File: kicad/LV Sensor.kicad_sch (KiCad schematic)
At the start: 69 parts, among them IC1 MCP2517FDT-H_SL, IC2 L78L05ABUTR, IC3 TLV74133PDBVR, IC4 TLV74125PDBVR, J1 Screw_Terminal_01x02, J16 USB_B_Micro, J2 Screw_Terminal_01x02, J3 Screw_Terminal_01x02, J4 Screw_Terminal_01x02, J5 Screw_Terminal_01x02, J6 Screw_Terminal_01x02, SW1 SW_Push, U0 AP63205WU-7, U10 MCP3204-CI/P, U2 XMSM0C1104SPW20R, U3 FT231XS-R, U6 DSC1001DL5-020.0000T, U7 ADS114S06BIPBSR, U8 LM2662MX/NOPB, U9 ATA6561-GAQW-N

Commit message: dfggd
fd
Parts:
- removed J6: Screw_Terminal_01x02, TerminalBlock_MetzConnect:TerminalBlock_MetzConnect_Type059_RT06302HBWC_1x02_P3.50mm_Horizontal, symbol Connector:Screw_Terminal_01x02
- added J6: 43650-0415, ADC2_AND_4:43650-04YY_151617, symbol LV-Sensor-Lib:43650-0415
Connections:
- net +12V: now also J6.1
- net GND: now also J6.2
- net CAN_L: now reaches U9.6 (CANL)
- net CAN_L: now also J6.4
- net CAN_H: now reaches U9.7 (CANH)
- net CAN_H: now also J6.3

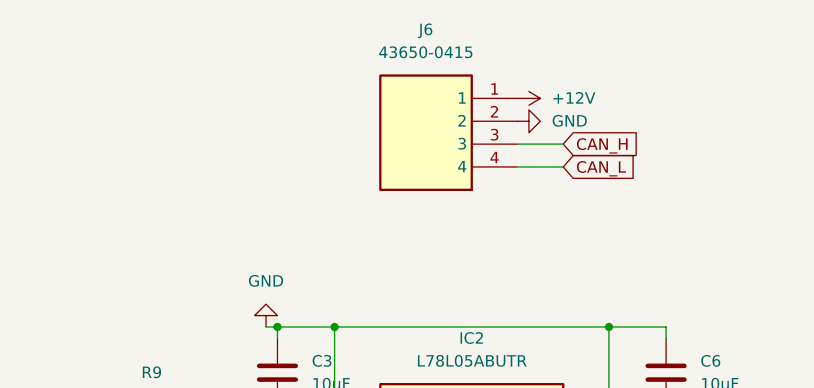
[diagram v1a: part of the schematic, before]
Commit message: fdg
dgf
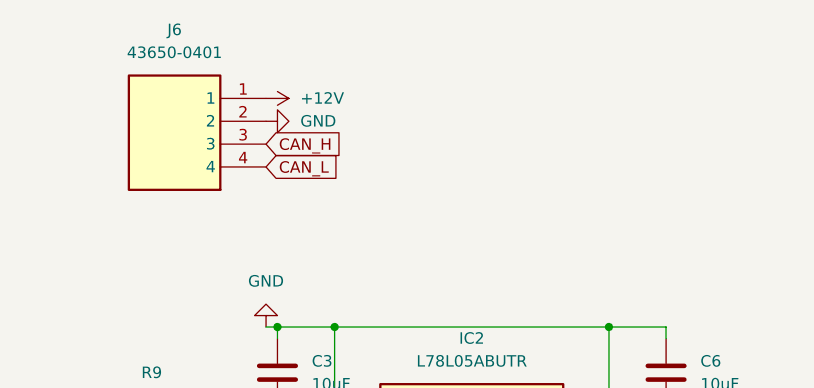
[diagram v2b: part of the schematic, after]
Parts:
- removed J6: 43650-0415, ADC2_AND_4:43650-04YY_151617, symbol LV-Sensor-Lib:43650-0415
- added J6: 43650-0401, ADC2_AND_4:43650-04YY_151617, symbol LV-Sensor-Lib:43650-0401
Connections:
- net +12V: now also J6.1
- net CAN_H: now also J6.3
- net CAN_L: now also J6.4
- net GND: now also J6.2
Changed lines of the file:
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@@
 	(wire
 		(pts
-			(xy 76.2 53.34) (xy 81.28 53.34)
-		)
-		(stroke
-			(width 0)
-			(type default)
-		)
-	)
-	(wire
-		(pts
 			(xy 276.86 73.66) (xy 270.51 73.66)
 		)
@@
 	(wire
 		(pts
-			(xy 76.2 55.88) (xy 81.28 55.88)
-		)
-		(stroke
-			(width 0)
-			(type default)
-		)
-	)
-	(wire
-		(pts
 			(xy 402.59 134.62) (xy 405.13 134.62)
 		)
@@
 	(global_label "CAN_H"
 		(shape input)
-		(at 81.28 53.34 0)
+		(at 48.26 53.34 0)
 		(fields_autoplaced yes)
 		(effects
@@
 		)
 		(property "Intersheetrefs" "${INTERSHEET_REFS}"
-			(at 90.2524 53.34 0)
+			(at 57.2324 53.34 0)
 			(effects
 				(font
@@
 	(global_label "CAN_L"
 		(shape input)
-		(at 81.28 55.88 0)
+		(at 397.51 68.58 0)
 		(fields_autoplaced yes)
 		(effects
@@
 		)
 		(property "Intersheetrefs" "${INTERSHEET_REFS}"
-			(at 89.95 55.88 0)
+			(at 406.18 68.58 0)
 			(effects
 				(font
@@
 	(global_label "CAN_L"
 		(shape input)
-		(at 397.51 68.58 0)
+		(at 48.26 55.88 0)
 		(fields_autoplaced yes)
 		(effects
@@
 		)
 		(property "Intersheetrefs" "${INTERSHEET_REFS}"
-			(at 406.18 68.58 0)
+			(at 56.93 55.88 0)
 			(effects
 				(font
@@
 	)
 	(symbol
-		(lib_id "LV-Sensor-Lib:43650-0415")
-		(at 76.2 55.88 180)
-		(unit 1)
-		(exclude_from_sim no)
-		(in_bom yes)
-		(on_board yes)
-		(dnp no)
-		(fields_autoplaced yes)
-		(property "Reference" "J6"
-			(at 66.04 40.64 0)
-			(effects
-				(font
-					(size 1.27 1.27)
-				)
-			)
-		)
-		(property "Value" "43650-0415"
-			(at 66.04 43.18 0)
-			(effects
-				(font
-					(size 1.27 1.27)
-				)
-			)
-		)
-		(property "Footprint" "ADC2_AND_4:43650-04YY_151617"
-			(at 59.69 -39.04 0)
-			(effects
-				(font
-					(size 1.27 1.27)
-				)
-				(justify left top)
-				(hide yes)
-			)
-		)
-		(property "Datasheet" "https://www.molex.com/pdm_docs/sd/436500215_sd.pdf"
-			(at 59.69 -139.04 0)
-			(effects
-				(font
-					(size 1.27 1.27)
-				)
-				(justify left top)
-				(hide yes)
-			)
-		)
-		(property "Description" "Micro-Fit 3.0 Vertical Header, 3.00mm Pitch, Single Row, 4 Circuits, with PCB Polarizing Peg, Glow-Wire Capable, Black"
-			(at 76.2 55.88 0)
-			(effects
-				(font
-					(size 1.27 1.27)
-				)
-				(hide yes)
-			)
-		)
-		(property "Height" "9.9"
-			(at 59.69 -339.04 0)
-			(effects
-				(font
-					(size 1.27 1.27)
-				)
-				(justify left top)
-				(hide yes)
-			)
-		)
-		(property "Mouser Part Number" "538-43650-0415"
-			(at 59.69 -439.04 0)
-			(effects
-				(font
-					(size 1.27 1.27)
-				)
-				(justify left top)
-				(hide yes)
-			)
-		)
-		(property "Mouser Price/Stock" "https://www.mouser.co.uk/ProductDetail/Molex/43650-0415?qs=GEJyObWCoZgrB2DNhHHwDQ%3D%3D"
-			(at 59.69 -539.04 0)
-			(effects
-				(font
-					(size 1.27 1.27)
-				)
-				(justify left top)
-				(hide yes)
-			)
-		)
-		(property "Manufacturer_Name" "Molex"
-			(at 59.69 -639.04 0)
-			(effects
-				(font
-					(size 1.27 1.27)
-				)
-				(justify left top)
-				(hide yes)
-			)
-		)
-		(property "Manufacturer_Part_Number" "43650-0415"
-			(at 59.69 -739.04 0)
-			(effects
-				(font
-					(size 1.27 1.27)
-				)
-				(justify left top)
-				(hide yes)
-			)
-		)
-		(pin "3"
-		)
-		(pin "4"
-		)
-		(pin "2"
-		)
-		(pin "1"
-		)
-		(instances
-			(project ""
-				(path "/1afce36f-b357-4e2a-9166-a84df6dcc281"
-					(reference "J6")
-					(unit 1)
-				)
-			)
-		)
-	)
-	(symbol
 		(lib_id "Device:C_Small")
 		(at 182.88 59.69 0)
@@
 	(symbol
 		(lib_id "power:+12V")
-		(at 76.2 48.26 270)
+		(at 48.26 48.26 270)
 		(unit 1)
 		(exclude_from_sim no)
@@
 		(on_board yes)
 		(dnp no)
-		(fields_autoplaced yes)
 		(property "Reference" "#PWR051"
-			(at 72.39 48.26 0)
+			(at 44.45 48.26 0)
 			(effects
 				(font
@@
 		)
 		(property "Value" "+12V"
-			(at 80.01 48.2599 90)
+			(at 52.07 48.2599 90)
 			(effects
 				(font
@@
 		)
 		(property "Footprint" ""
-			(at 76.2 48.26 0)
+			(at 48.26 48.26 0)
 			(effects
 				(font
@@
 		)
 		(property "Datasheet" ""
-			(at 76.2 48.26 0)
+			(at 48.26 48.26 0)
 			(effects
 				(font
@@
 		)
 		(property "Description" "Power symbol creates a global label with name \"+12V\""
-			(at 76.2 48.26 0)
+			(at 48.26 48.26 0)
 			(effects
 				(font
@@
 		)
 		(instances
-			(project ""
+			(project "LV Sensor"
 				(path "/1afce36f-b357-4e2a-9166-a84df6dcc281"
 					(reference "#PWR051")
@@
 	(symbol
 		(lib_id "power:GND")
-		(at 76.2 50.8 90)
+		(at 48.26 50.8 90)
 		(unit 1)
 		(exclude_from_sim no)
@@
 		(fields_autoplaced yes)
 		(property "Reference" "#PWR052"
-			(at 82.55 50.8 0)
+			(at 54.61 50.8 0)
 			(effects
 				(font
@@
 		)
 		(property "Value" "GND"
-			(at 80.01 50.7999 90)
+			(at 52.07 50.7999 90)
 			(effects
 				(font
@@
 		)
 		(property "Footprint" ""
-			(at 76.2 50.8 0)
+			(at 48.26 50.8 0)
 			(effects
 				(font
@@
 		)
 		(property "Datasheet" ""
-			(at 76.2 50.8 0)
+			(at 48.26 50.8 0)
 			(effects
 				(font
@@
 		)
 		(property "Description" "Power symbol creates a global label with name \"GND\" , ground"
-			(at 76.2 50.8 0)
+			(at 48.26 50.8 0)
 			(effects
 				(font
@@
 		)
 		(instances
-			(project ""
+			(project "LV Sensor"
 				(path "/1afce36f-b357-4e2a-9166-a84df6dcc281"
 					(reference "#PWR052")
@@
 					(unit 1)
 				)
+			)
+		)
+	)
+	(symbol
+		(lib_id "LV-Sensor-Lib:43650-0401")
+		(at 48.26 55.88 180)
+		(unit 1)
+		(exclude_from_sim no)
+		(in_bom yes)
+		(on_board yes)
+		(dnp no)
+		(fields_autoplaced yes)
+		(property "Reference" "J6"
+			(at 38.1 40.64 0)
+			(effects
+				(font
+					(size 1.27 1.27)
+				)
+			)
+		)
+		(property "Value" "43650-0401"
+			(at 38.1 43.18 0)
+			(effects
+				(font
+					(size 1.27 1.27)
+				)
+			)
+		)
+		(property "Footprint" "ADC2_AND_4:43650-04YY_151617"
+			(at 31.75 -39.04 0)
+			(effects
+				(font
+					(size 1.27 1.27)
+				)
+				(justify left top)
+				(hide yes)
+			)
+		)
+		(property "Datasheet" "https://www.molex.com/pdm_docs/sd/436500200_sd.pdf"
+			(at 31.75 -139.04 0)
+			(effects
+				(font
+					(size 1.27 1.27)
+				)
+				(justify left top)
+				(hide yes)
+			)
+		)
+		(property "Description" "Micro-Fit 3.0 Right-Angle Header, 3.00mm Pitch, Single Row, 4 Circuits, with Snap-in Plastic Peg PCB Lock, Glow-Wire Capable, Black"
+			(at 48.26 55.88 0)
+			(effects
+				(font
+					(size 1.27 1.27)
+				)
+				(hide yes)
+			)
+		)
+		(property "Height" "5.57"
+			(at 31.75 -339.04 0)
+			(effects
+				(font
+					(size 1.27 1.27)
+				)
+				(justify left top)
+				(hide yes)
+			)
+		)
+		(property "Mouser Part Number" "538-43650-0401"
+			(at 31.75 -439.04 0)
+			(effects
+				(font
+					(size 1.27 1.27)
+				)
+				(justify left top)
+				(hide yes)
+			)
+		)
+		(property "Mouser Price/Stock" "https://www.mouser.co.uk/ProductDetail/Molex/43650-0401?qs=tCVB0Dok1YBvOr8VX%2FzPCg%3D%3D"
+			(at 31.75 -539.04 0)
+			(effects
+				(font
+					(size 1.27 1.27)
+				)
+				(justify left top)
+				(hide yes)
+			)
+		)
+		(property "Manufacturer_Name" "Molex"
+			(at 31.75 -639.04 0)
+			(effects
+				(font
+					(size 1.27 1.27)
+				)
+				(justify left top)
+				(hide yes)
+			)
+		)
+		(property "Manufacturer_Part_Number" "43650-0401"
+			(at 31.75 -739.04 0)
+			(effects
+				(font
+					(size 1.27 1.27)
+				)
+				(justify left top)
+				(hide yes)
+			)
+		)
+		(pin "4"
+		)
+		(pin "1"
+		)
+		(pin "3"
+		)
+		(pin "2"
+		)
+		(instances
+			(project ""
+				(path "/1afce36f-b357-4e2a-9166-a84df6dcc281"
+					(reference "J6")
+					(unit 1)
+				)
